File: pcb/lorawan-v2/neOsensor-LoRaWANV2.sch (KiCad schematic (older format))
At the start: 29 parts, among them J1 Conn_01x04, J2 Conn_01x02, J3 Conn_01x04, J4 Conn_01x04, J5 Conn_01x05, J6 Conn_01x05, J7 Conn_01x05, SW1 G71Y, U1 OLED1.3_I2C, U2 ATECC508A, U3 AMS1117-3.3, U4 HTCC-AB01

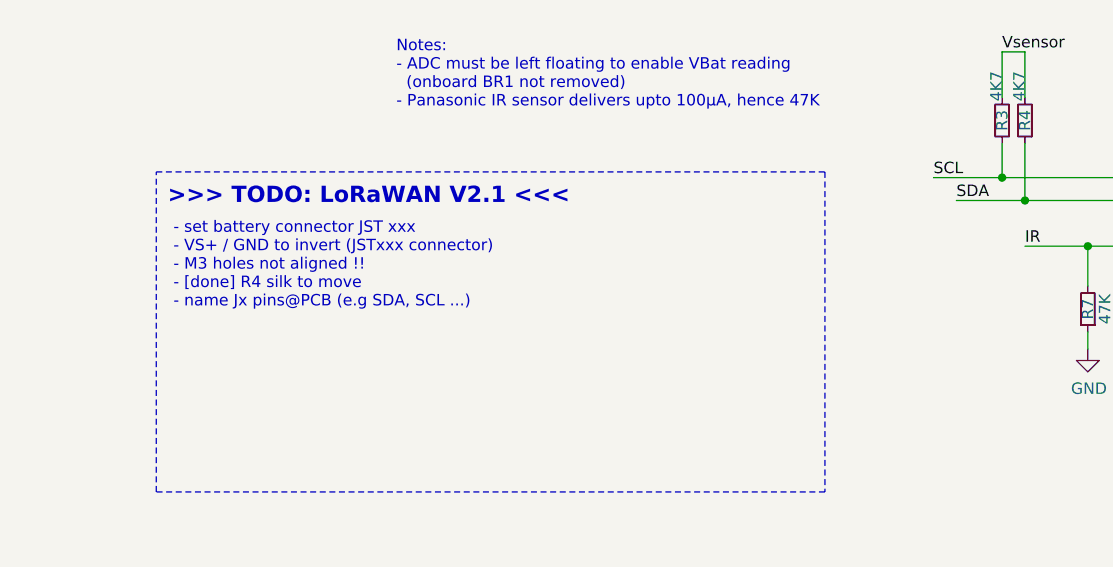
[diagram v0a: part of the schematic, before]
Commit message: update
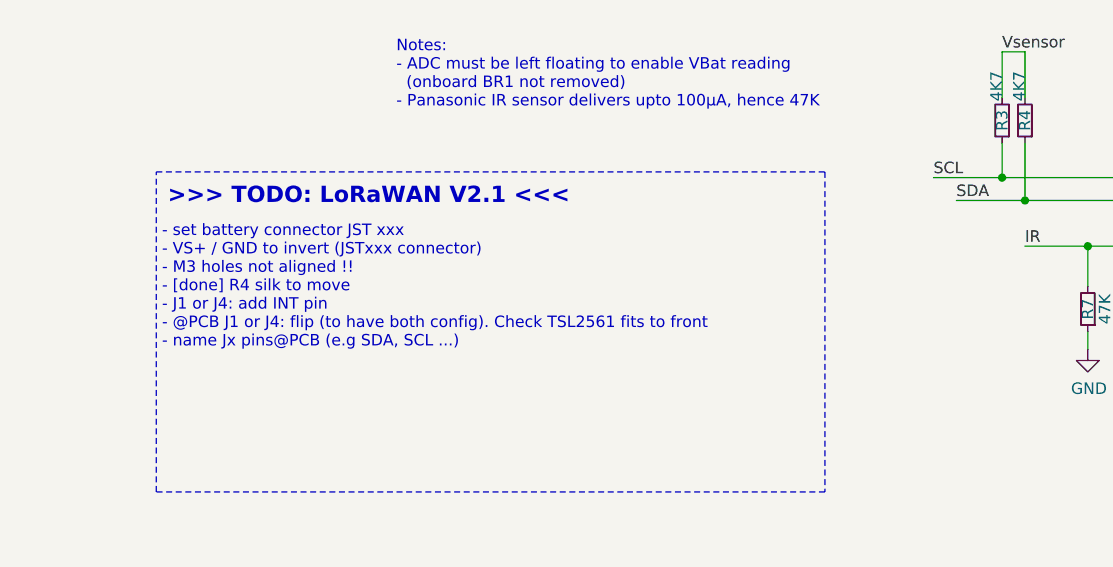
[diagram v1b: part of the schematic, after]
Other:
- note added: "- set battery connector JST xxx\n- VS+ / GND to invert (JSTxxx connector)\n- M3 holes not aligned !!\n- [done] R4 silk to move\n- J1 or J4: add INT pin\n- @PCB J1 or J4: flip (to have both config). Check TSL2561 fits to front\n- name Jx pins@PCB (e.g SDA, SCL ...)"
- note removed: "- set battery connector JST xxx\n- VS+ / GND to invert (JSTxxx connector)\n- M3 holes not aligned !!\n- [done] R4 silk to move\n- name Jx pins@PCB (e.g SDA, SCL ...)"
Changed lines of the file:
@@
 Text Notes 3250 3025 0    71   ~ 14
 >>> TODO: LoRaWAN V2.1 <<<
-Text Notes 3275 3475 0    50   ~ 0
-- set battery connector JST xxx\n- VS+ / GND to invert (JSTxxx connector)\n- M3 holes not aligned !!\n- [done] R4 silk to move\n- name Jx pins@PCB (e.g SDA, SCL ...)
+Text Notes 3225 3650 0    50   ~ 0
+- set battery connector JST xxx\n- VS+ / GND to invert (JSTxxx connector)\n- M3 holes not aligned !!\n- [done] R4 silk to move\n- J1 or J4: add INT pin\n- @PCB J1 or J4: flip (to have both config). Check TSL2561 fits to front\n- name Jx pins@PCB (e.g SDA, SCL ...)
 $EndSCHEMATC
